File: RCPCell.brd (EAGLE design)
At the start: 99.8 x 44.5 mm, 27 parts, among them IC1 SIM900, U1 PESDXS4UD, U7 FAN8303

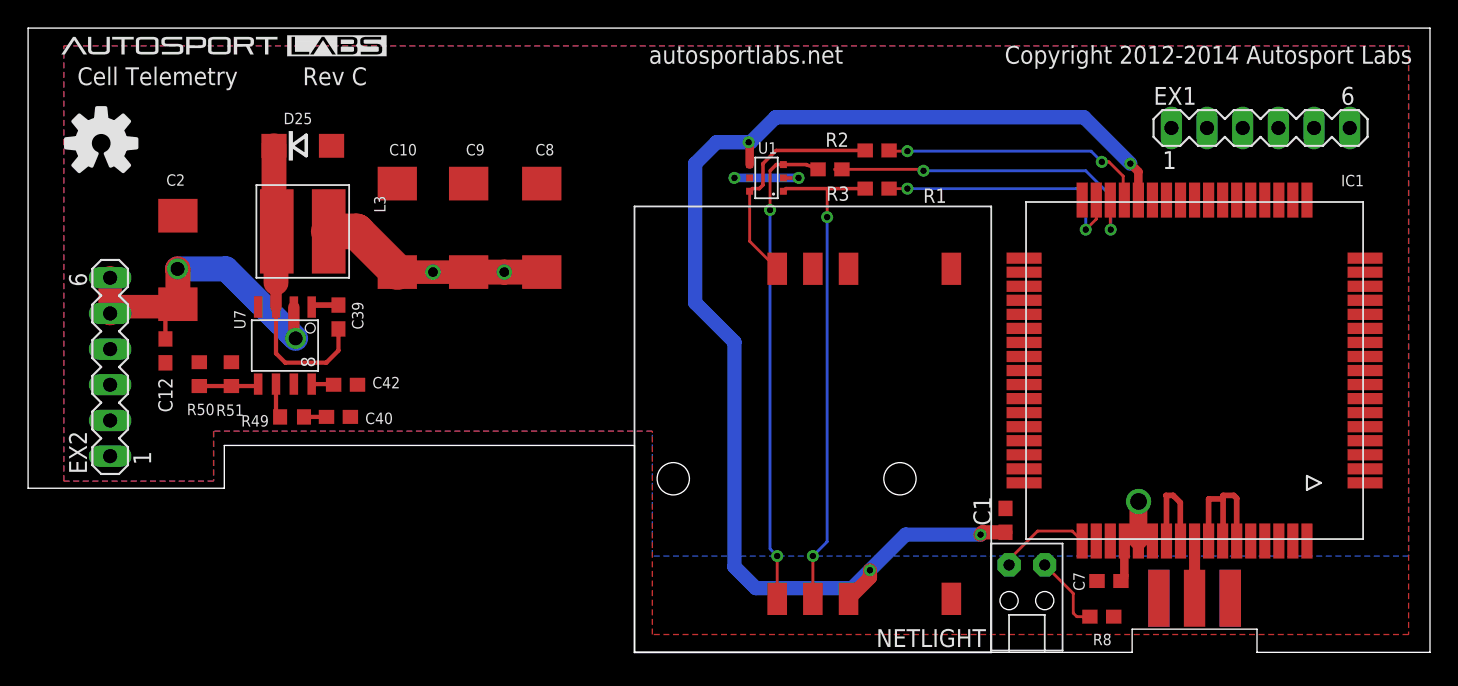
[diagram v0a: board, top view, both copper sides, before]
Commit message: tentative final version of RevC module
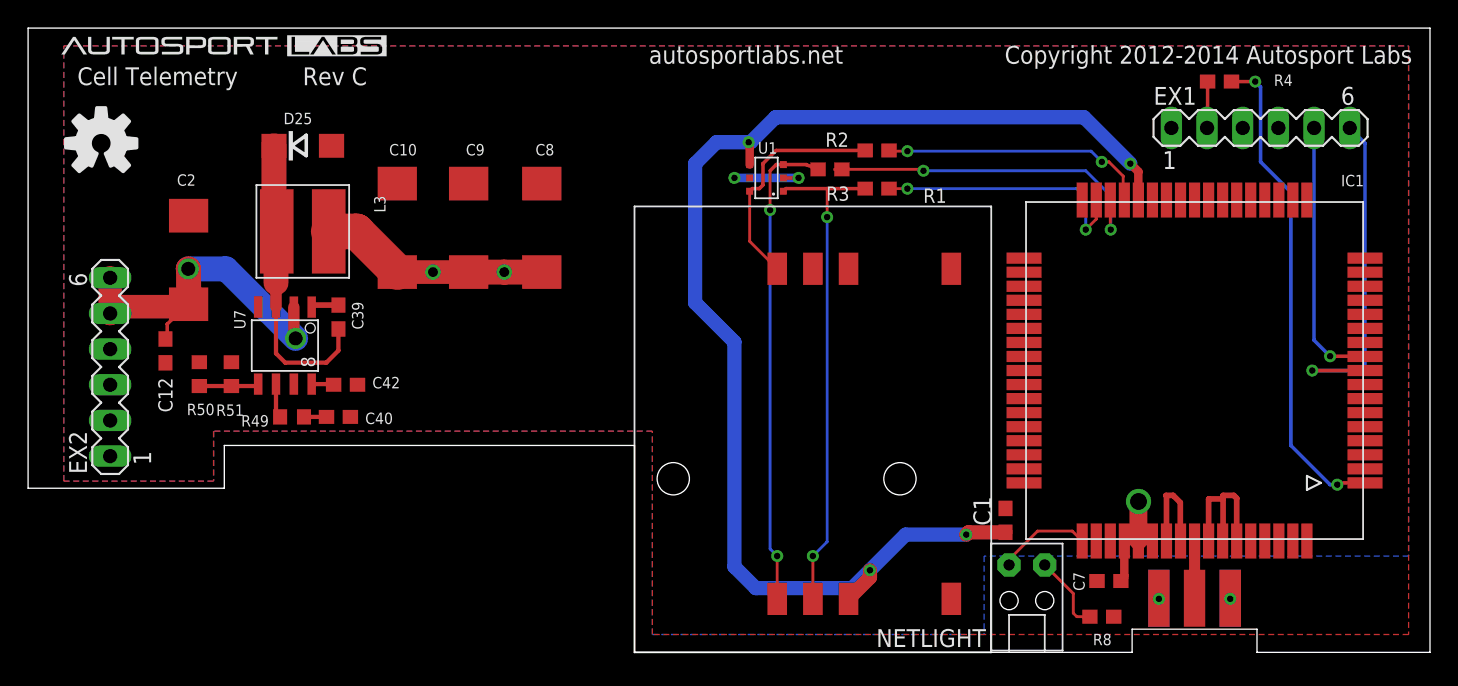
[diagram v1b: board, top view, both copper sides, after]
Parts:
- added R4: 1k, SparkFun:0603
- moved C2 0.76 mm to (11.4, 27.9)
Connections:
- removed net +5V: EX2.3, EX2.4
- removed net PWRKEY_OUT: IC1.2
- removed net RXD3: EX1.6
- removed net TXD3: EX1.5
- new net EXT_CTRL: EX1.2, R4.2
- net DIN: now also EX1.5
- net DOUT: now also EX1.6
- net PWRKEY: now also R4.1
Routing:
- net PWRKEY: track 0.00 -> 35.1 mm, vias 0 -> 2
- net DOUT: track 0.00 -> 25.2 mm, vias 0 -> 1
- net DIN: track 0.00 -> 19.2 mm, vias 0 -> 1
- net EXT_CTRL: track 0.00 -> 3.32 mm
- net SAFE12V: track 24.4 -> 26.0 mm
- net GND: vias 2 -> 4
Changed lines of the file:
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@@
 </element>
 <element name="L3" library="sumida_inductors" package="CD54" value="CD54" x="19.558" y="29.972" rot="R270"/>
-<element name="C2" library="rcl" package="SMC_D" value="47uF" x="10.668" y="27.94" smashed="yes" rot="R90">
-<attribute name="NAME" x="11.176" y="34.036" size="0.8128" layer="25" rot="R180"/>
+<element name="C2" library="rcl" package="SMC_D" value="47uF" x="11.43" y="27.94" smashed="yes" rot="R90">
+<attribute name="NAME" x="11.938" y="34.036" size="0.8128" layer="25" rot="R180"/>
+</element>
+<element name="R4" library="SparkFun" package="0603" value="1k" x="84.836" y="40.64" smashed="yes" rot="R180">
+<attribute name="NAME" x="90.043" y="41.148" size="0.8128" layer="25" font="vector" rot="R180"/>
 </element>
 </elements>
@@
 <contactref element="C2" pad="-"/>
 <contactref element="C12" pad="2"/>
-<wire x1="85.598" y1="3.8481" x2="85.598" y2="3.8481" width="0" layer="19" extent="1-16"/>
-<wire x1="80.518" y1="3.8481" x2="80.518" y2="3.8481" width="0" layer="19" extent="1-16"/>
+<via x="80.518" y="3.81" extent="1-16" drill="0.4572"/>
+<via x="85.598" y="3.81" extent="1-16" drill="0.4572"/>
+<wire x1="80.518" y1="3.8481" x2="80.518" y2="3.81" width="0.254" layer="16"/>
+<wire x1="85.598" y1="3.8481" x2="85.598" y2="3.81" width="0.254" layer="16"/>
 </signal>
 <signal name="DIN">
 <contactref element="IC1" pad="10"/>
+<contactref element="EX1" pad="5"/>
+<wire x1="95.197" y1="21.066" x2="95.181" y2="21.082" width="0.254" layer="1"/>
+<wire x1="95.181" y1="21.082" x2="92.71" y2="21.082" width="0.254" layer="1"/>
+<via x="92.71" y="21.082" extent="1-16" drill="0.4572"/>
+<wire x1="92.71" y1="21.082" x2="91.567" y2="22.225" width="0.254" layer="16"/>
+<wire x1="91.567" y1="22.225" x2="91.567" y2="37.338" width="0.254" layer="16"/>
 </signal>
 <signal name="DOUT">
 <contactref element="IC1" pad="9"/>
+<contactref element="EX1" pad="6"/>
+<wire x1="94.107" y1="37.338" x2="95.197" y2="36.248" width="0.254" layer="16"/>
+<wire x1="95.197" y1="36.248" x2="95.197" y2="20.066" width="0.254" layer="16"/>
+<wire x1="95.197" y1="20.066" x2="91.44" y2="20.066" width="0.254" layer="16"/>
+<via x="91.44" y="20.066" extent="1-16" drill="0.4572"/>
+<wire x1="91.44" y1="20.066" x2="95.197" y2="20.066" width="0.254" layer="1"/>
 </signal>
 <signal name="V+" class="1">
@@
 <contactref element="IC1" pad="57"/>
 <contactref element="IC1" pad="56"/>
-<wire x1="36.7284" y1="27.0764" x2="36.703" y2="27.1018" width="1.778" layer="1"/>
 <wire x1="78.058" y1="5.326" x2="78.058" y2="7.927" width="0.6096" layer="1"/>
 <via x="79.0702" y="10.7442" extent="1-16" drill="1.2"/>
 <polygon width="0.4064" layer="16">
-<vertex x="44.45" y="6.858"/>
+<vertex x="44.45" y="1.27"/>
 <vertex x="44.45" y="15.748"/>
 <vertex x="13.208" y="15.748"/>
@@
 <vertex x="98.298" y="43.18"/>
 <vertex x="98.298" y="6.858"/>
+<vertex x="68.072" y="6.858"/>
+<vertex x="68.072" y="1.27"/>
 </polygon>
 <wire x1="79.0702" y1="10.7442" x2="79.058" y2="10.732" width="0.8128" layer="1"/>
@@
 <wire x1="23.393" y1="29.972" x2="26.289" y2="27.076" width="2.54" layer="1"/>
 <wire x1="78.058" y1="5.326" x2="77.812" y2="5.08" width="0" layer="19" extent="1-1"/>
-<wire x1="36.7284" y1="27.0764" x2="36.576" y2="27.076" width="0" layer="19" extent="1-1"/>
-</signal>
-<signal name="+5V">
-<contactref element="EX2" pad="3"/>
-<contactref element="EX2" pad="4"/>
-<wire x1="5.842" y1="19.05" x2="5.842" y2="21.59" width="0" layer="19" extent="1-1"/>
 </signal>
 <signal name="RF_ANT">
@@
 <signal name="PWRKEY">
 <contactref element="IC1" pad="1"/>
-</signal>
-<signal name="PWRKEY_OUT">
-<contactref element="IC1" pad="2"/>
+<contactref element="R4" pad="1"/>
+<wire x1="85.686" y1="40.64" x2="87.376" y2="40.64" width="0.254" layer="1"/>
+<via x="87.376" y="40.64" extent="1-16" drill="0.4572"/>
+<wire x1="87.376" y1="40.64" x2="87.757" y2="40.259" width="0.254" layer="16"/>
+<wire x1="87.757" y1="40.259" x2="87.757" y2="34.925" width="0.254" layer="16"/>
+<wire x1="87.757" y1="34.925" x2="89.916" y2="32.766" width="0.254" layer="16"/>
+<wire x1="89.916" y1="32.766" x2="89.916" y2="14.732" width="0.254" layer="16"/>
+<wire x1="89.916" y1="14.732" x2="92.71" y2="11.938" width="0.254" layer="16"/>
+<wire x1="92.71" y1="11.938" x2="93.218" y2="11.938" width="0.254" layer="16"/>
+<via x="93.218" y="11.938" extent="1-16" drill="0.4572"/>
+<wire x1="93.218" y1="11.938" x2="93.346" y2="12.066" width="0.254" layer="1"/>
+<wire x1="93.346" y1="12.066" x2="95.197" y2="12.066" width="0.254" layer="1"/>
 </signal>
 <signal name="STATUS">
@@
 <via x="59.944" y="5.842" extent="1-16" drill="0.4572"/>
 <wire x1="59.944" y1="5.842" x2="62.484" y2="8.382" width="1.016" layer="16"/>
-<wire x1="62.484" y1="8.382" x2="67.818" y2="8.382" width="1.016" layer="16"/>
-<via x="67.818" y="8.382" extent="1-16" drill="0.4572"/>
-<wire x1="67.818" y1="8.382" x2="67.984" y2="8.548" width="1.016" layer="1"/>
-<wire x1="67.984" y1="8.548" x2="69.596" y2="8.548" width="1.016" layer="1"/>
+<wire x1="62.484" y1="8.382" x2="66.802" y2="8.382" width="1.016" layer="16"/>
+<via x="66.802" y="8.382" extent="1-16" drill="0.4572"/>
+<wire x1="66.802" y1="8.382" x2="66.968" y2="8.548" width="1.016" layer="1"/>
+<wire x1="66.968" y1="8.548" x2="69.596" y2="8.548" width="1.016" layer="1"/>
 <wire x1="79.058" y1="32.205" x2="79.058" y2="34.226" width="0.6096" layer="1"/>
 <wire x1="79.058" y1="34.226" x2="78.486" y2="34.798" width="0.6096" layer="1"/>
@@
 <wire x1="5.842" y1="24.13" x2="5.842" y2="26.67" width="1.6764" layer="1"/>
 <wire x1="5.842" y1="24.13" x2="6.325" y2="24.613" width="1.6764" layer="1"/>
-<wire x1="6.325" y1="24.613" x2="9.906" y2="24.613" width="1.6764" layer="1"/>
-<wire x1="9.779" y1="22.313" x2="9.779" y2="24.486" width="0.3048" layer="1"/>
-<wire x1="9.779" y1="24.486" x2="9.906" y2="24.613" width="0.3048" layer="1"/>
+<wire x1="6.325" y1="24.613" x2="10.668" y2="24.613" width="1.6764" layer="1"/>
+<wire x1="10.541" y1="24.486" x2="10.668" y2="24.613" width="0.3048" layer="1"/>
 <contactref element="U7" pad="2"/>
 <contactref element="C2" pad="+"/>
-<wire x1="10.668" y1="24.79" x2="10.668" y2="27.2796" width="1.778" layer="1"/>
-<wire x1="10.668" y1="27.2796" x2="10.6426" y2="27.305" width="1.778" layer="1"/>
-<via x="10.6426" y="27.305" extent="1-16" drill="1"/>
-<wire x1="10.6426" y1="27.305" x2="14.097" y2="27.305" width="1.778" layer="16"/>
+<wire x1="11.43" y1="24.79" x2="11.43" y2="27.2796" width="1.778" layer="1"/>
+<wire x1="11.43" y1="27.2796" x2="11.4046" y2="27.305" width="1.778" layer="1"/>
+<via x="11.4046" y="27.305" extent="1-16" drill="1"/>
+<wire x1="11.4046" y1="27.305" x2="14.097" y2="27.305" width="1.778" layer="16"/>
 <wire x1="14.097" y1="27.305" x2="19.05" y2="22.352" width="1.778" layer="16"/>
 <via x="19.05" y="22.352" extent="1-16" drill="1"/>
 <wire x1="19.05" y1="22.352" x2="18.923" y2="22.479" width="0.8128" layer="1"/>
 <wire x1="18.923" y1="22.479" x2="18.923" y2="24.5872" width="0.8128" layer="1"/>
-<wire x1="9.906" y1="24.613" x2="10.668" y2="24.79" width="0" layer="19" extent="1-1"/>
-</signal>
-<signal name="TXD3">
-<contactref element="EX1" pad="5"/>
-</signal>
-<signal name="RXD3">
-<contactref element="EX1" pad="6"/>
+<wire x1="9.779" y1="22.313" x2="9.906" y2="22.44" width="0.254" layer="1"/>
+<wire x1="9.906" y1="22.44" x2="9.906" y2="23.368" width="0.254" layer="1"/>
+<wire x1="9.906" y1="23.368" x2="11.151" y2="24.613" width="0.254" layer="1"/>
+<wire x1="11.328" y1="24.79" x2="11.43" y2="24.79" width="0.254" layer="1"/>
+<wire x1="11.328" y1="24.79" x2="11.151" y2="24.613" width="0.254" layer="1"/>
+<wire x1="11.151" y1="24.613" x2="10.668" y2="24.613" width="0.254" layer="1"/>
 </signal>
 <signal name="USB_DM_HS_OUT">
@@
 <contactref element="R50" pad="1"/>
 </signal>
+<signal name="EXT_CTRL">
+<contactref element="EX1" pad="2"/>
+<contactref element="R4" pad="2"/>
+<wire x1="83.947" y1="37.338" x2="83.986" y2="37.377" width="0.254" layer="1"/>
+<wire x1="83.986" y1="37.377" x2="83.986" y2="40.64" width="0.254" layer="1"/>
+</signal>
 </signals>

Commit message: yak shaving design a bit
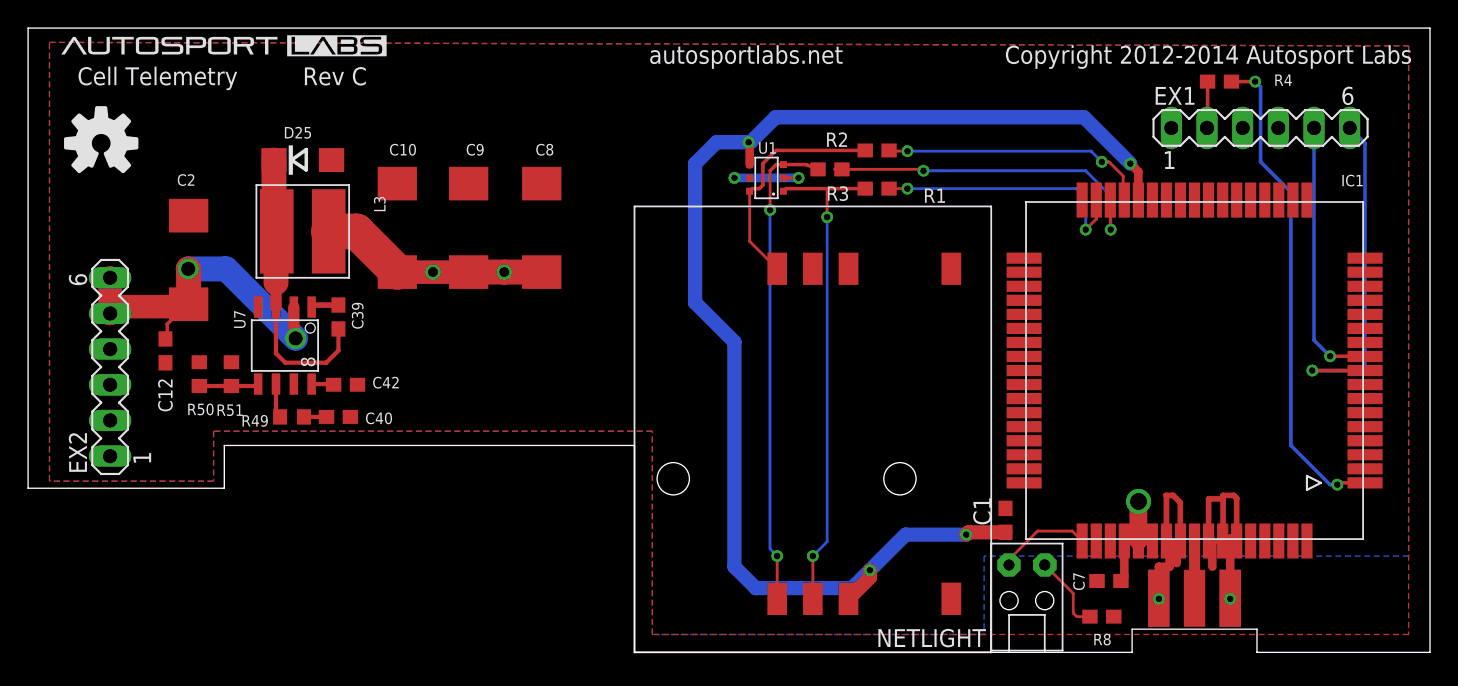
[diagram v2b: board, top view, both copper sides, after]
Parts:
- R51: value 2.43K 1% -> 3.9K 1%
- moved D25 1.02 mm to (19.6, 35.1)
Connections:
- net GND renamed N$2
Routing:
- net N$2: track 24.3 -> 34.7 mm
- net N$1000: track 21.5 -> 20.5 mm
